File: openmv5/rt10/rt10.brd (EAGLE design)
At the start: 35.6 x 44.5 mm, 222 parts, among them CN1 S2B-PH-K-S(LF)(SN), IC1 LM66200DRLR, IC2 AP61300Z6-7, IC3 IS42S16160G-6BL, IC4 ATECC608B-MAHDA-T, IC5 IS25LP064D-JKLE-TR, IC6 IS25LP128F-JKLE-TR, IC7 MXC4005XC, IC8 MIMXRT1052DVL6B, IC9 KSZ8081RNDCA-TR, J1 USB4105-GF-A, J2 DNP, J3 DNP, J4 DF12-36-DS, J5 USD-1040310811, J6 DNP, J7 DNP, J8 3221-10-0300-00, M1 9774030151R, M2 9774030151R, Q1 2N7002KW_R1_00001, Q2 2N7002KW_R1_00001, Q3 2N7002KW_R1_00001, Q4 2N7002KW_R1_00001, Q5 2N7002KW_R1_00001, Q6 PMXB120EPEZ, U1 MIC5365-3.3YMT-TZ, U2 BQ24075RGTR, U3 LBEE5KL1DX-883, Y1 SC32S-7PF20PPM, Y2 XRCGB24M000F3M00R0

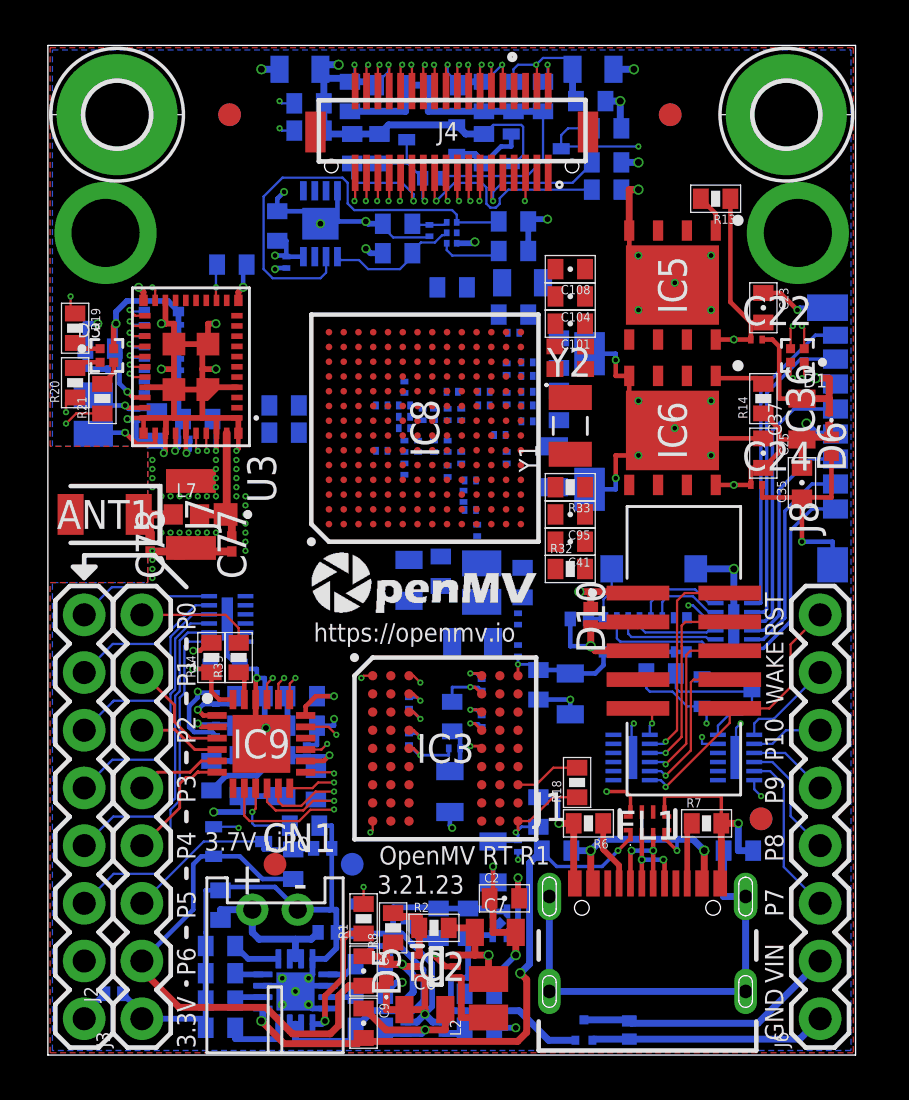
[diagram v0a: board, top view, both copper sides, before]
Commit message: Final
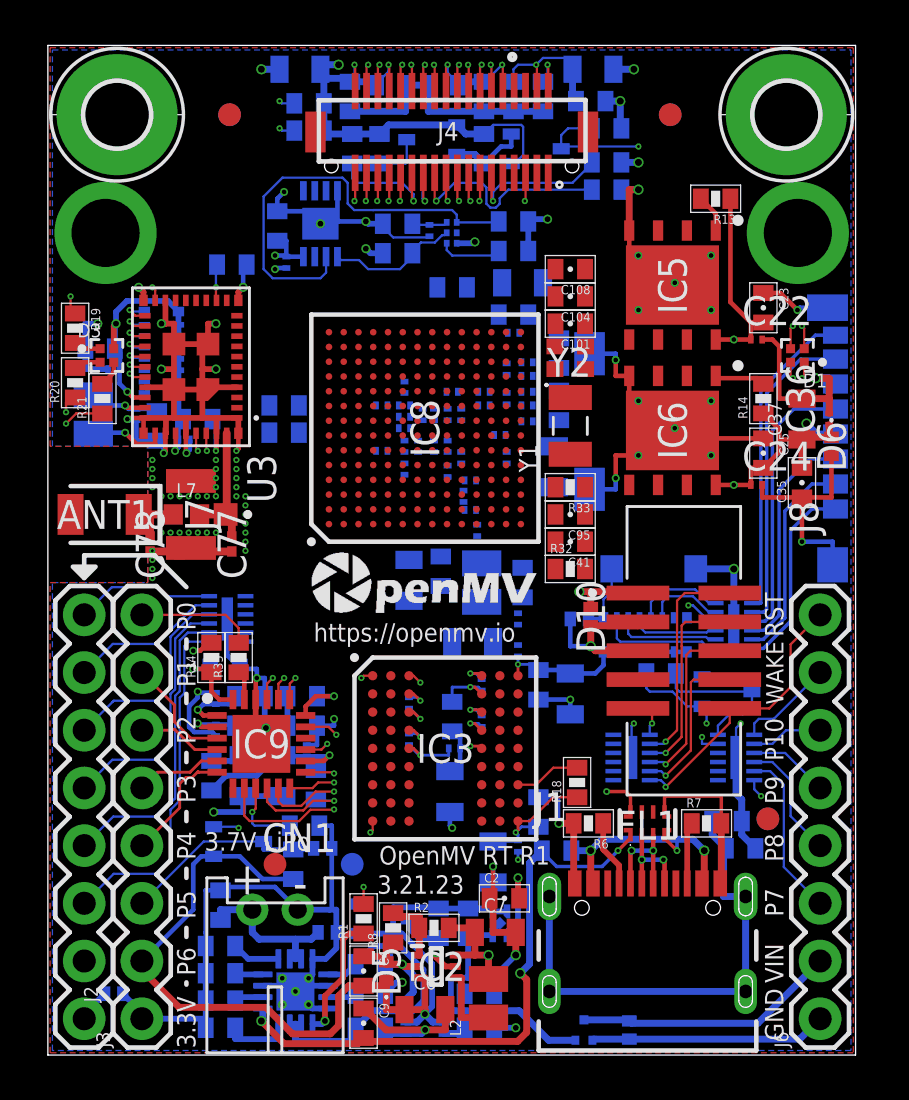
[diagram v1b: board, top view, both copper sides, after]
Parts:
- removed D11: CPDQT5V0HE-HF, CPDQT5V0HE-HF:CPDQT5V0HEHF
- removed L3: 100, sfe:C0402
- added C110: 1nF, sfe:0402-CAP
- added R41: 1M, sfe:0402-RES
- moved FD2 0.30 mm to (31.7, 10.4)
- moved FD4 0.30 mm to (31.7, 10.4)
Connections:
- net DCMI_FSIN: no longer D11.1
- net GND: now also C110.1, R41.2; no longer D11.2, L3.1
- net SHELL_GND: now also C110.2, R41.1; no longer L3.2
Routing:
- net GND: track 253.8 -> 248.6 mm, vias 102 -> 101
- net SHELL_GND: track 20.0 -> 21.6 mm
- net DCMI_FSIN: track 5.55 -> 4.33 mm
